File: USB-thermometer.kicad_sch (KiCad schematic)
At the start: 3 parts, among them J1 USB_A, J2 Conn_01x04_Pin, U1 Seeed Studio XIAO SAMD21

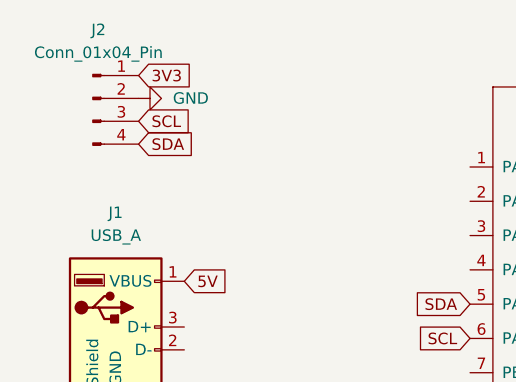
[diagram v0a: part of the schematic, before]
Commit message: finished design and generated gerber
finished design and generated gerber
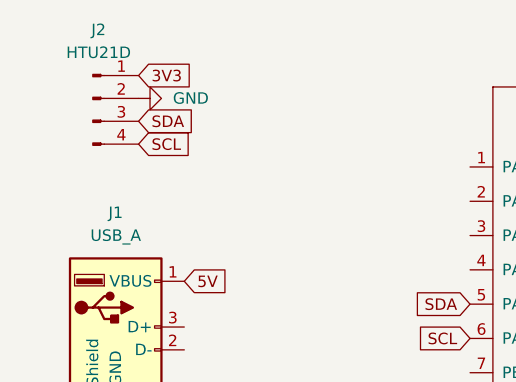
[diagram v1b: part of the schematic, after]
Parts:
- J2: value Conn_01x04_Pin -> HTU21D
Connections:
- net SCL: now also J2.4 (Pin_4); no longer J2.3 (Pin_3)
- net SDA: now also J2.3 (Pin_3); no longer J2.4 (Pin_4)
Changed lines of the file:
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@@
+		)
+	)
+	(global_label "SDA"
+		(shape input)
+		(at 88.9 54.61 0)
+		(fields_autoplaced yes)
+		(effects
+			(font
+				(size 1.27 1.27)
+			)
+			(justify left)
+		)
+		(property "Intersheetrefs" "${INTERSHEET_REFS}"
+			(at 95.4533 54.61 0)
+			(effects
+				(font
+					(size 1.27 1.27)
+				)
+				(justify left)
+				(hide yes)
+			)
 		)
 	)
@@
 		)
 	)
+	(global_label "3V3"
+		(shape input)
+		(at 167.64 67.31 0)
+		(fields_autoplaced yes)
+		(effects
+			(font
+				(size 1.27 1.27)
+			)
+			(justify left)
+		)
+		(property "Intersheetrefs" "${INTERSHEET_REFS}"
+			(at 174.1328 67.31 0)
+			(effects
+				(font
+					(size 1.27 1.27)
+				)
+				(justify left)
+				(hide yes)
+			)
+		)
+	)
 	(global_label "SCL"
 		(shape input)
-		(at 88.9 54.61 0)
+		(at 88.9 57.15 0)
 		(fields_autoplaced yes)
 		(effects
@@
 		)
 		(property "Intersheetrefs" "${INTERSHEET_REFS}"
-			(at 95.3928 54.61 0)
-			(effects
-				(font
-					(size 1.27 1.27)
-				)
-				(justify left)
-				(hide yes)
-			)
-		)
-	)
-	(global_label "SDA"
-		(shape input)
-		(at 88.9 57.15 0)
-		(fields_autoplaced yes)
-		(effects
-			(font
-				(size 1.27 1.27)
-			)
-			(justify left)
-		)
-		(property "Intersheetrefs" "${INTERSHEET_REFS}"
-			(at 95.4533 57.15 0)
-			(effects
-				(font
-					(size 1.27 1.27)
-				)
-				(justify left)
-				(hide yes)
-			)
-		)
-	)
-	(global_label "3V3"
-		(shape input)
-		(at 167.64 67.31 0)
-		(fields_autoplaced yes)
-		(effects
-			(font
-				(size 1.27 1.27)
-			)
-			(justify left)
-		)
-		(property "Intersheetrefs" "${INTERSHEET_REFS}"
-			(at 174.1328 67.31 0)
+			(at 95.3928 57.15 0)
 			(effects
 				(font
@@
 			)
 		)
-		(property "Value" "Conn_01x04_Pin"
+		(property "Value" "HTU21D"
 			(at 84.455 46.99 0)
 			(effects
